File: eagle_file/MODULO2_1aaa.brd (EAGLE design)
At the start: 160 x 100 mm, 59 parts, among them IC1 74HC595N

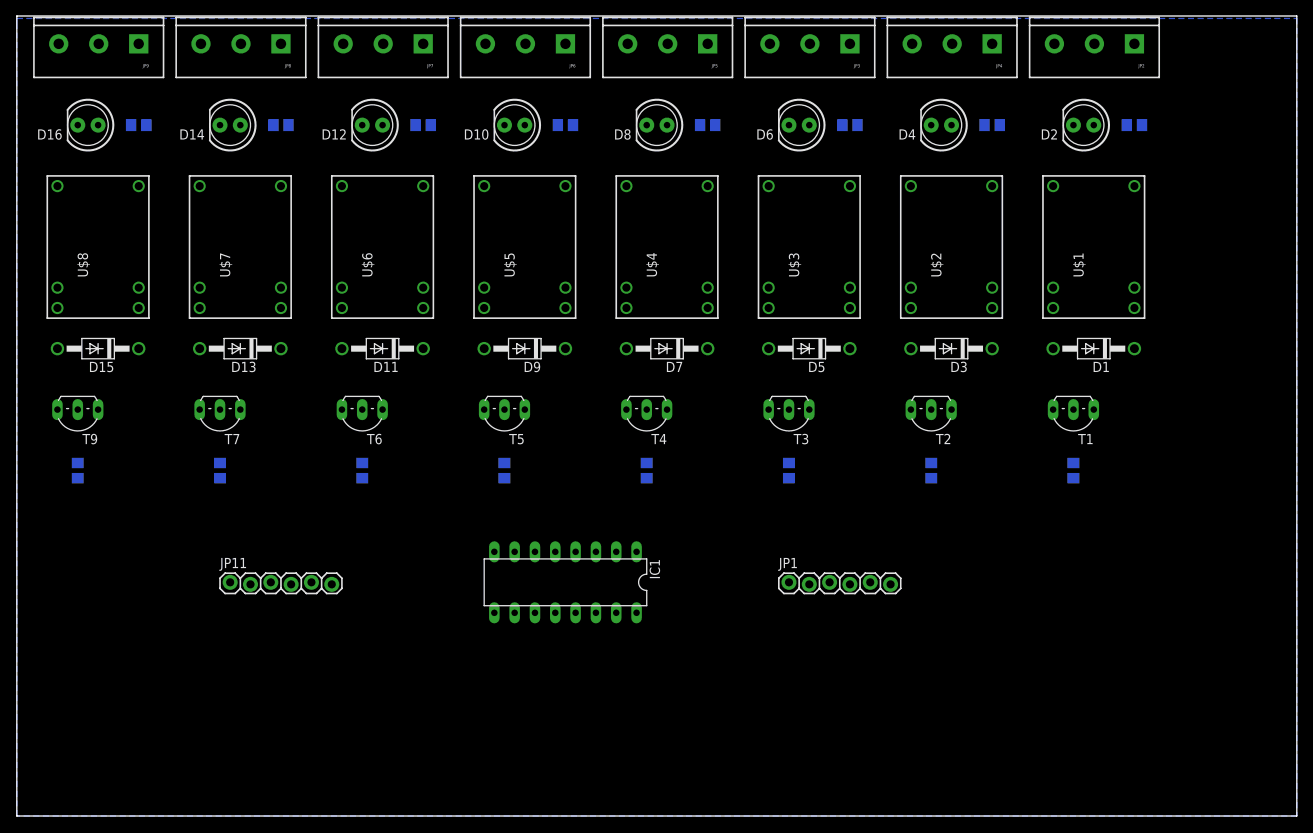
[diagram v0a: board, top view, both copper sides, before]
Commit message: MODULO2_def
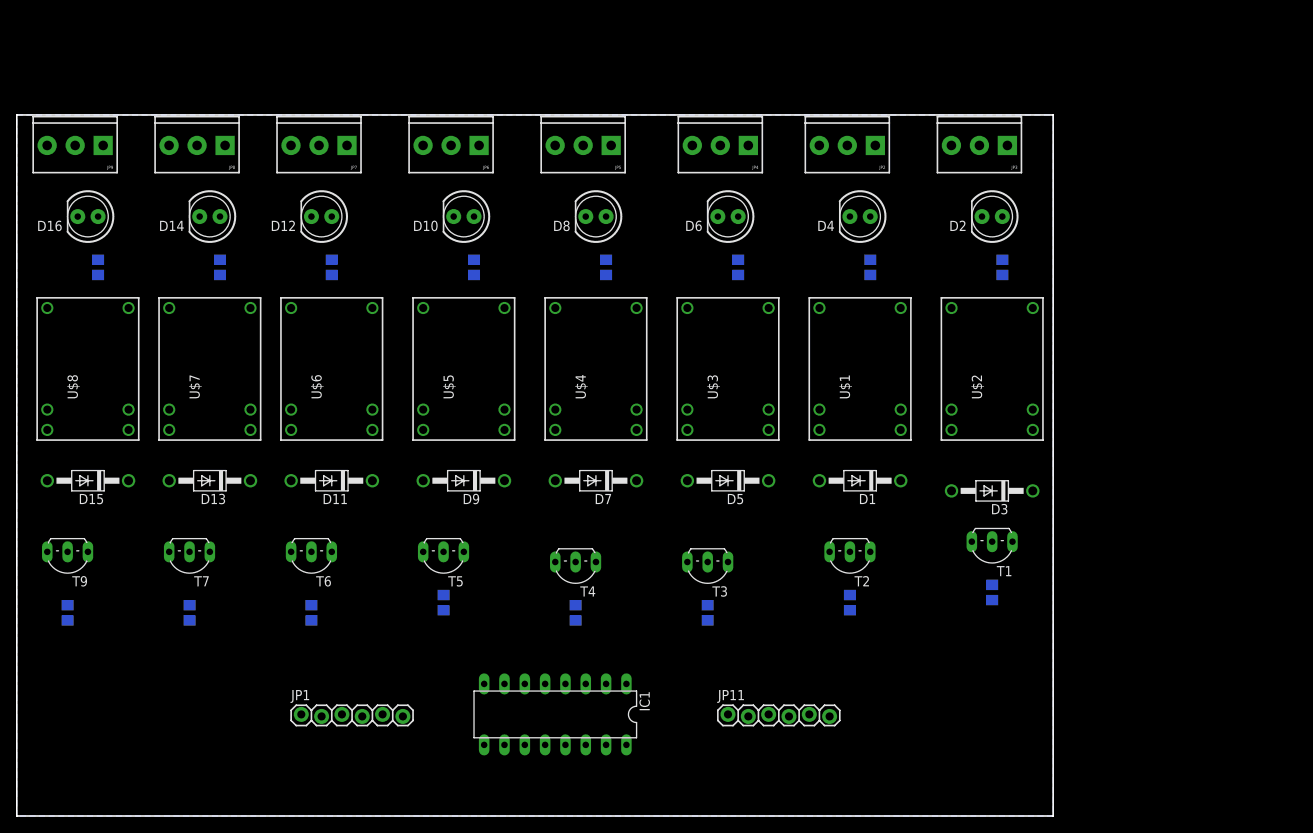
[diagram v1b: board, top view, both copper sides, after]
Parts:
- JP2, JP3, JP4, JP5, JP6, JP7, JP8, JP9: device SparkFun-Connectors:SCREWTERMINAL-5MM-3 -> SparkFun-Connectors:SCREWTERMINAL-3.5MM-3
- moved JP11 64.4 mm to (88.9, 12.7)
- moved JP1 63.2 mm to (35.6, 12.7)
- moved JP2 34.8 mm to (107.3, 83.8)
- moved D1 33.6 mm to (105.4, 41.9)
- moved JP4 33.0 mm to (91.4, 83.8)
- moved U$1 32.9 mm to (105.4, 55.9)
- moved R2 24.3 mm to (123.2, 68.6), turned to 270 degrees
- moved JP3 23.4 mm to (123.8, 83.8)
- moved R4 23.4 mm to (106.7, 68.6), turned to 270 degrees
- moved R6 22.6 mm to (90.2, 68.6), turned to 270 degrees
- moved R8 21.8 mm to (73.7, 68.6), turned to 270 degrees
- moved T3 21.6 mm to (86.4, 30.5)
- moved R10 21.1 mm to (57.1, 68.6), turned to 270 degrees
- moved R12 21.1 mm to (39.4, 68.6), turned to 270 degrees
- moved T4 21.0 mm to (69.8, 30.5)
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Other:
- board size 160 x 100 mm -> 129.5 x 87.6 mm
